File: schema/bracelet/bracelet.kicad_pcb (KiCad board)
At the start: 2 copper layers, 40 x 32.8 mm, 12 parts, among them J1 IN+, J2 B+, J3 IN-, J4 B-, U1 ESP32-C3, U2 AUIPS1051L, U3 BMI270

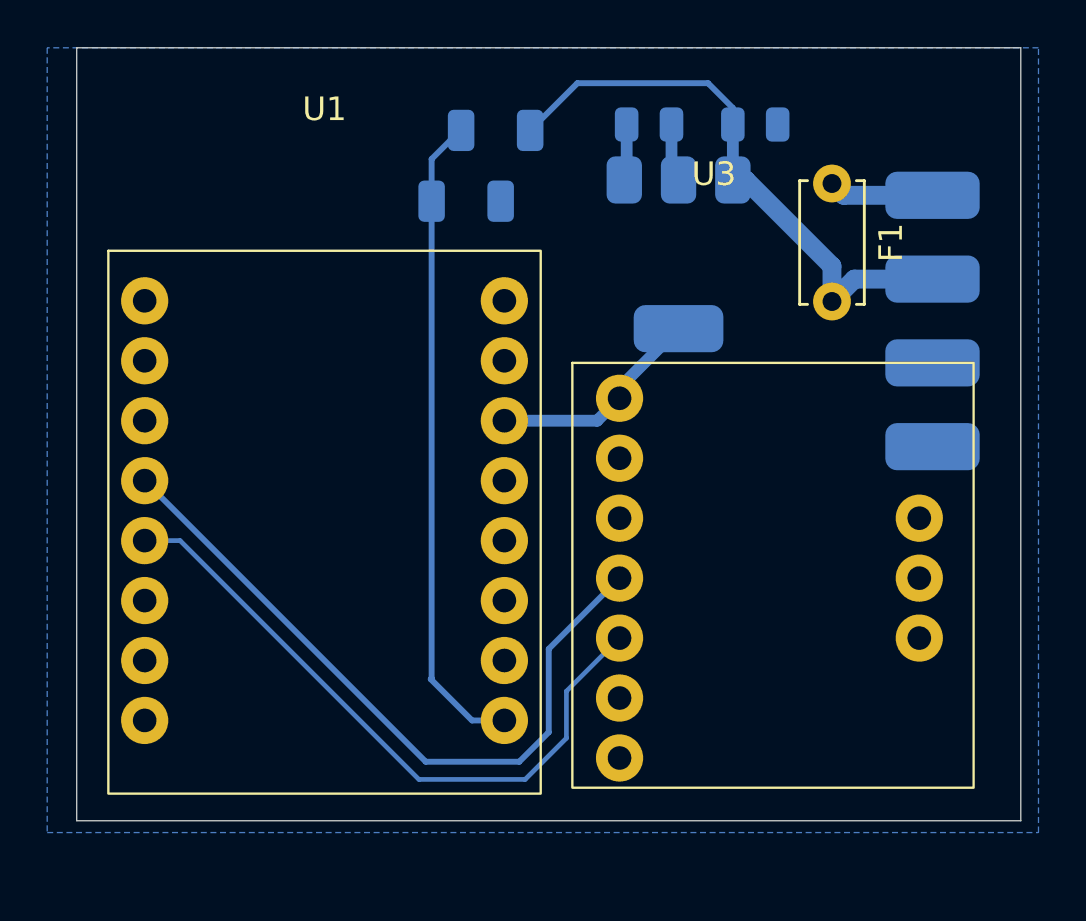
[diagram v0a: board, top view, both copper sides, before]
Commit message: Update Architecture db
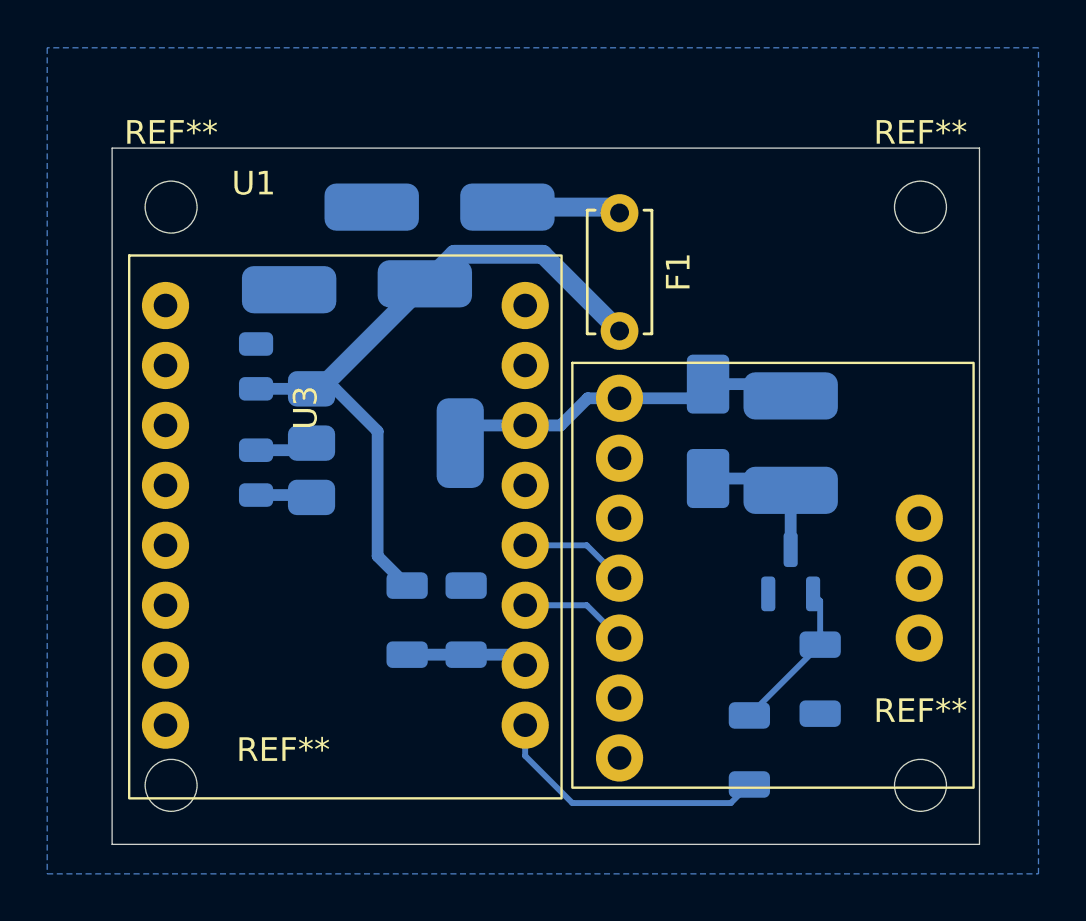
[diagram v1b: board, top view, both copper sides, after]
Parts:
- added D1: 1N5819, Diode_SMD:D_SMA, B.Cu at (179.8, 112.5)
- added J5: Vib+, Connector_Wire:SolderWirePad_1x01_SMD_2x4mm, B.Cu at (183.2, 111.0)
- added J6: Vib-, Connector_Wire:SolderWirePad_1x01_SMD_2x4mm, B.Cu at (183.2, 115.0)
- added Q1: AO3400A, Package_TO_SOT_SMD:SOT-23, B.Cu at (183.2, 118.5)
- added R3: 100, Resistor_SMD:R_1206_3216Metric, B.Cu at (181.5, 126.0)
- added R4: 100k, Resistor_SMD:R_1206_3216Metric, B.Cu at (184.5, 123.0)
- added REF**: MountingHole_2.2mm_M2, MountingHole:MountingHole_2.2mm_M2, F.Cu at (157.0, 127.5)
- added REF**: MountingHole_2.2mm_M2, MountingHole:MountingHole_2.2mm_M2, F.Cu at (157.0, 103.0)
- added REF**: MountingHole_2.2mm_M2, MountingHole:MountingHole_2.2mm_M2, F.Cu at (188.8, 103.0)
- added REF**: MountingHole_2.2mm_M2, MountingHole:MountingHole_2.2mm_M2, F.Cu at (188.8, 127.5)
- moved J4 28.1 mm to (162.0, 106.5)
- moved J3 24.7 mm to (165.5, 103.0)
- moved C2 23.5 mm to (160.6, 109.8), turned to 90 degrees
- moved C1 22.2 mm to (160.6, 114.2), turned to -90 degrees
- moved J2 21.5 mm to (167.8, 106.2)
- moved R1 21.1 mm to (167.0, 120.5), turned to -90 degrees
- moved J1 18.0 mm to (171.2, 103.0)
- moved R2 17.8 mm to (169.5, 120.5), turned to -90 degrees
- moved U2 14.8 mm to (166.1, 113.0), turned to 0 degrees
- moved F1 9.09 mm to (176.0, 103.2)
- moved U1 0.91 mm to (164.4, 99.5)
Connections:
- R1 pad 2: Net-(U1-IO0) -> Net-(U1-IO1)
- R2 pad 2: Net-(U1-IO0) -> Net-(U1-IO1)
- U1 pad 1: unconnected-(U1-IO1-Pad1) -> Net-(U1-IO1)
- U1 pad 2: unconnected-(U1-IO2-Pad2) -> Net-(U1-IO2)
- U1 pad 3: unconnected-(U1-IO3-Pad3) -> Net-(U1-IO3)
- U1 pad 8: Net-(U1-IO8) -> unconnected-(U1-IO8-Pad8)
- U1 pad 9: Net-(U1-IO9) -> unconnected-(U1-IO9-Pad9)
- U3 pad 4: Net-(U1-IO8) -> Net-(U1-IO3)
- U3 pad 5: Net-(U1-IO9) -> Net-(U1-IO2)
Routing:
- net Net-(U1-IO8): track 31.8 -> 0.00 mm
- net Net-(U1-IO9): track 28.0 -> 0.00 mm
- net Net-(U1-IO0): track 27.7 -> 12.0 mm
- net Net-(Q1-G): track 0.00 -> 6.52 mm
- net Net-(D1-A): track 0.00 -> 6.36 mm
- net +3.3V: track 11.8 -> 17.8 mm
- net Net-(U1-IO1): track 0.00 -> 5.24 mm
- net Net-(J2-Pin_1): track 24.8 -> 29.7 mm
- net Net-(U1-IO3): track 0.00 -> 4.57 mm
- net Net-(U1-IO2): track 0.00 -> 4.57 mm
- net unconnected-(U1-IO8-Pad8): track 0.00 -> 0.75 mm
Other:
- board size 40 x 32.8 mm -> 36.8 x 29.5 mm
